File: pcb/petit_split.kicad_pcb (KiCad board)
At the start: 2 copper layers, 67.8 x 48.2 mm, 18 parts, among them J2 LED, SW1 KEY_SWITCH, SW2 KEY_SWITCH, SW3 KEY_SWITCH, SW4 KEY_SWITCH, U1 ProMicro

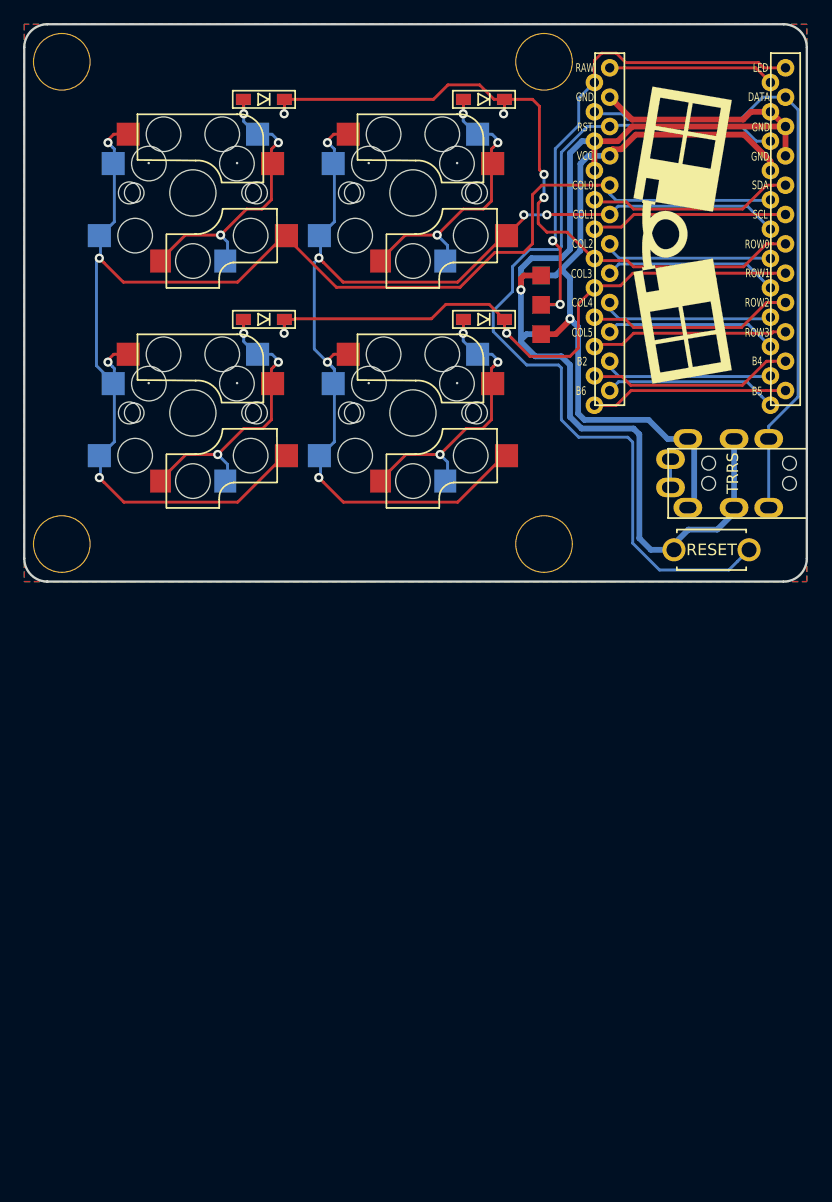
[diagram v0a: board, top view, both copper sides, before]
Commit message: Add imposition
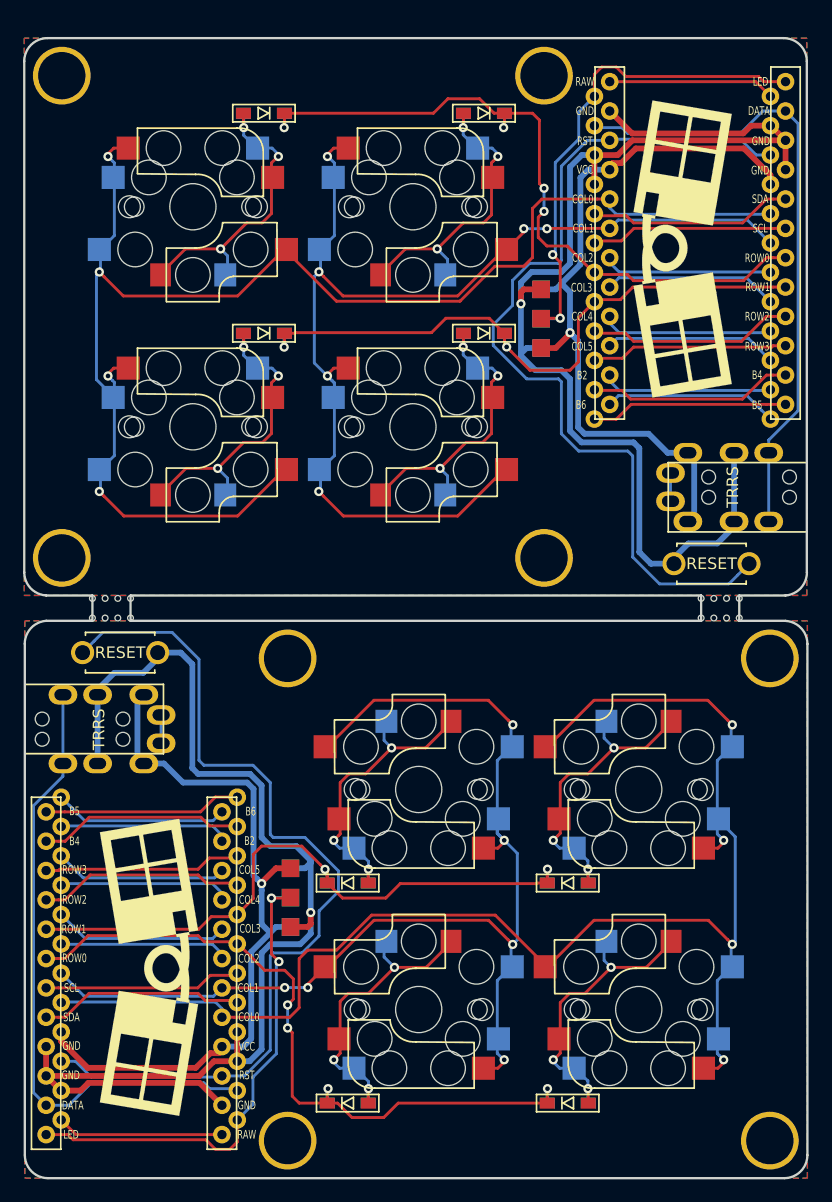
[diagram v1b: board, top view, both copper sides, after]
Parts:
- removed the SW1 at (61.9, 70.6)
- added D1: D, kbd:D3_SMD, F.Cu at (94.3, 149.4)
- added D2: D, kbd:D3_SMD, F.Cu at (75.2, 149.4)
- added D3: D, kbd:D3_SMD, F.Cu at (94.3, 130.3)
- added D4: D, kbd:D3_SMD, F.Cu at (75.2, 130.3)
- added G***: LOGO, kbd:petit_split-logo, F.Cu at (58.0, 137.7)
- added G***: LOGO, kbd:petit_split-logo, B.Cu at (58.0, 137.7)
- added J2: LED, kbd:StripLED_rev, F.Cu at (70.3, 134.2)
- added Ref**: Val**, kbd:IM_HOLE, F.Cu at (105.8, 107.4)
- added Ref**: Val**, kbd:IM_HOLE, F.Cu at (55.4, 107.4)
- added Ref**: Val**, kbd:IM_HOLE, F.Cu at (54.2, 107.4)
- added Ref**: Val**, kbd:IM_HOLE, F.Cu at (109.2, 107.4)
- added Ref**: Val**, kbd:IM_HOLE, F.Cu at (109.2, 105.7)
- added Ref**: Val**, kbd:IM_HOLE, F.Cu at (105.8, 105.7)
- added Ref**: Val**, kbd:IM_HOLE, F.Cu at (108.0, 105.7)
- added Ref**: Val**, kbd:IM_HOLE, F.Cu at (107.0, 105.7)
- added Ref**: Val**, kbd:IM_HOLE, F.Cu at (54.2, 105.7)
- added Ref**: Val**, kbd:IM_HOLE, F.Cu at (55.4, 105.7)
- added Ref**: Val**, kbd:IM_HOLE, F.Cu at (53.1, 105.7)
- added Ref**: Val**, kbd:IM_HOLE, F.Cu at (107.0, 107.4)
- added Ref**: Val**, kbd:IM_HOLE, F.Cu at (56.5, 105.7)
- added Ref**: Val**, kbd:IM_HOLE, F.Cu at (108.0, 107.4)
- added Ref**: Val**, kbd:HOLE, F.Cu at (111.8, 152.7)
- added Ref**: Val**, kbd:HOLE, F.Cu at (111.8, 110.9)
- added Ref**: Val**, kbd:HOLE, F.Cu at (70.0, 152.7)
- added Ref**: Val**, kbd:HOLE, F.Cu at (70.0, 110.9)
- added Ref**: Val**, kbd:IM_HOLE, F.Cu at (56.5, 107.4)
- added Ref**: Val**, kbd:IM_HOLE, F.Cu at (53.1, 107.4)
- added SW1: KEY_SWITCH, kbd:CherryMX_KailhLowProfile_Hotswap_rev1, F.Cu at (100.5, 141.3)
- added SW1: KEY_SWITCH, kbd:CherryMX_KailhLowProfile_Hotswap_rev1, F.Cu at (61.9, 71.8)
- added SW2: KEY_SWITCH, kbd:CherryMX_KailhLowProfile_Hotswap_rev1, F.Cu at (81.4, 141.3)
- added SW3: KEY_SWITCH, kbd:CherryMX_KailhLowProfile_Hotswap_rev1, F.Cu at (100.5, 122.2)
- added SW4: KEY_SWITCH, kbd:CherryMX_KailhLowProfile_Hotswap_rev1, F.Cu at (81.4, 122.2)
- added SW5: , kbd:ResetSW, F.Cu at (55.5, 110.4)
- added TRRS: MJ-4PP-9, kbd:MJ-4PP-9, F.Cu at (47.3, 116.2)
- added U1: ProMicro, kbd:ProMicro_v2, F.Cu at (56.8, 137.7)
- SW2, SW3, SW4: footprint kbd:CherryMX_KailhLowProfile_Hotswap -> kbd:CherryMX_KailhLowProfile_Hotswap_rev1
- moved D1 1.20 mm to (68.0, 63.7)
- moved D2 1.20 mm to (87.0, 63.7)
- moved D3 1.20 mm to (68.0, 82.8)
- moved D4 1.20 mm to (87.0, 82.8)
- moved G*** 1.20 mm to (104.2, 75.5) (x2)
- moved J2 1.20 mm to (92.0, 79.0)
- moved Ref** 1.20 mm to (92.2, 102.2)
- moved Ref** 1.20 mm to (92.2, 60.5)
- moved Ref** 1.20 mm to (50.5, 102.2)
- moved Ref** 1.20 mm to (50.5, 60.5)
- moved SW2 1.20 mm to (80.9, 71.8)
- moved SW5 1.20 mm to (106.8, 102.7)
- moved TRRS 1.20 mm to (115.0, 97.0)
- moved U1 1.20 mm to (105.5, 75.5)
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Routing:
- net col0: track 126.0 -> 252.0 mm, vias 4 -> 8
- net GND: track 108.1 -> 216.1 mm, vias 1 -> 2
- net col1: track 100.3 -> 200.6 mm, vias 6 -> 12
- net reset: track 78.2 -> 156.5 mm
- net VCC: track 65.8 -> 131.6 mm, vias 1 -> 2
- net row0: track 63.0 -> 126.0 mm, vias 4 -> 8
- net row1: track 56.1 -> 112.2 mm, vias 2 -> 4
- net data: track 54.7 -> 109.3 mm
- net led: track 43.5 -> 87.1 mm, vias 2 -> 4
- net Net-(D2-Pad2): track 26.9 -> 53.8 mm, vias 3 -> 6
- net Net-(D3-Pad2): track 26.8 -> 53.7 mm, vias 3 -> 6
- net Net-(D1-Pad2): track 26.8 -> 53.5 mm, vias 3 -> 6
- net Net-(D4-Pad2): track 26.7 -> 53.5 mm, vias 3 -> 6
- net Net-(U1-Pad9): track 17.8 -> 35.6 mm
- net Net-(U1-Pad11): track 17.7 -> 35.5 mm
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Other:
- board size 67.8 x 48.2 mm -> 67.8 x 98.7 mm
